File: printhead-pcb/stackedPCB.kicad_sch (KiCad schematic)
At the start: 5 parts, among them J13 Steckverbinder_Male_1

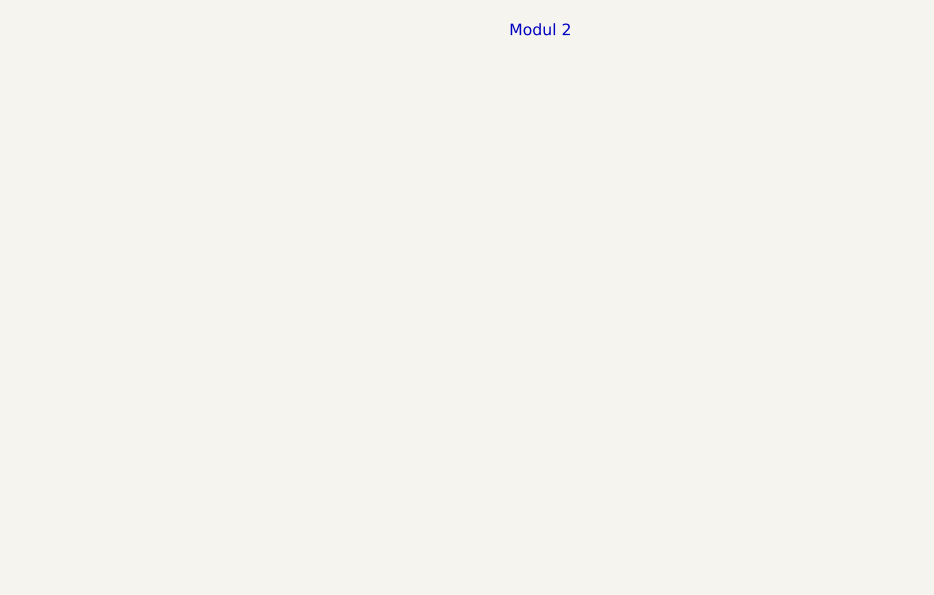
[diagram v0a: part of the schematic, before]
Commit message: prepared second module for tomorrow
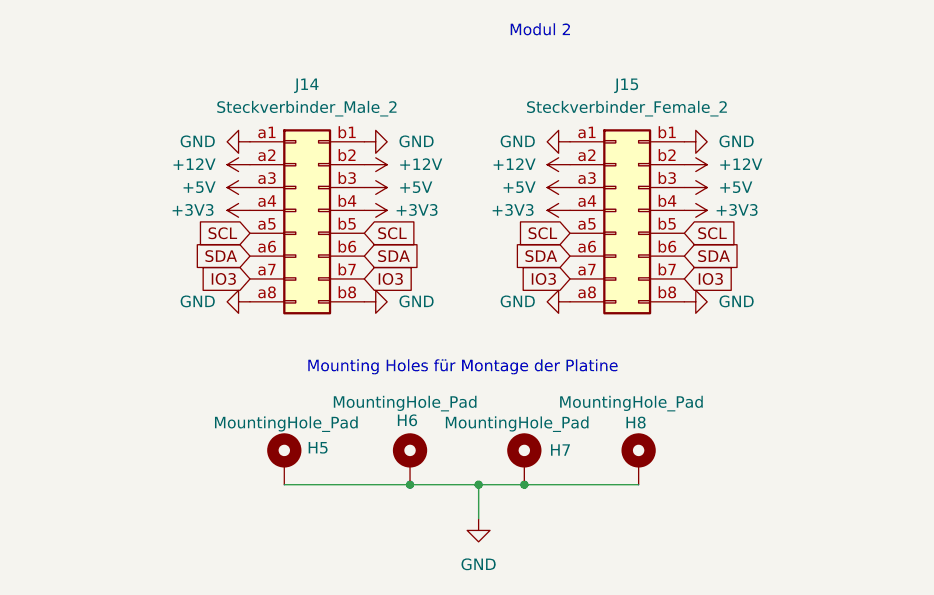
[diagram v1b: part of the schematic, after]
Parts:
- added H5, H6, H7, H8: MountingHole_Pad, MountingHole:MountingHole_2.2mm_M2_Pad_TopBottom, symbol Mechanical:MountingHole_Pad
- added J14: Steckverbinder_Male_2, CustomFotLibByJan:BF100-16-A-D-1-0640-L-C, symbol Connector_Generic:Conn_02x08_Row_Letter_First
- added J15: Steckverbinder_Female_2, CustomFotLibByJan:BF100-16-A-D-1-0640-L-C, symbol Connector_Generic:Conn_02x08_Row_Letter_First
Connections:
- net +12V: now also J14.a2 (Pin_a2), J14.b2 (Pin_b2), J15.a2 (Pin_a2), J15.b2 (Pin_b2)
- net +3V3: now also J14.a4 (Pin_a4), J14.b4 (Pin_b4), J15.a4 (Pin_a4), J15.b4 (Pin_b4)
- net +5V: now also J14.a3 (Pin_a3), J14.b3 (Pin_b3), J15.a3 (Pin_a3), J15.b3 (Pin_b3)
- net GND: now also H5.1, H6.1, H7.1, H8.1, J14.a1 (Pin_a1), J14.a8 (Pin_a8), J14.b1 (Pin_b1), J14.b8 (Pin_b8), J15.a1 (Pin_a1), J15.a8 (Pin_a8), J15.b1 (Pin_b1), J15.b8 (Pin_b8)
- net IO3: now also J14.a7 (Pin_a7), J14.b7 (Pin_b7), J15.a7 (Pin_a7), J15.b7 (Pin_b7)
- net SCL: now also J14.a5 (Pin_a5), J14.b5 (Pin_b5), J15.a5 (Pin_a5), J15.b5 (Pin_b5)
- net SDA: now also J14.a6 (Pin_a6), J14.b6 (Pin_b6), J15.a6 (Pin_a6), J15.b6 (Pin_b6)

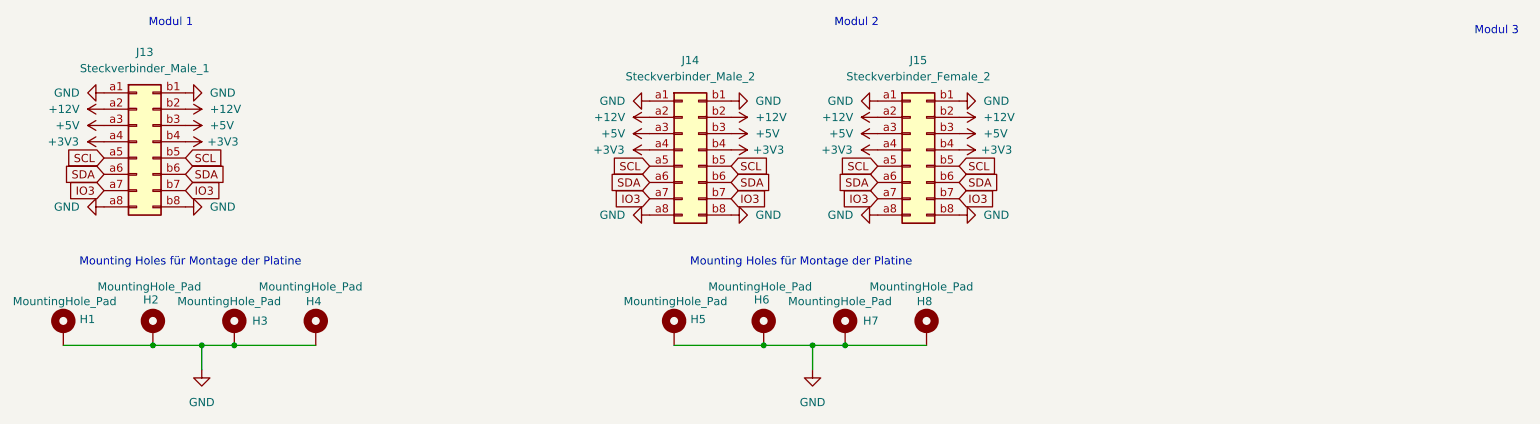
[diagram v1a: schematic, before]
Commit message: refractoring
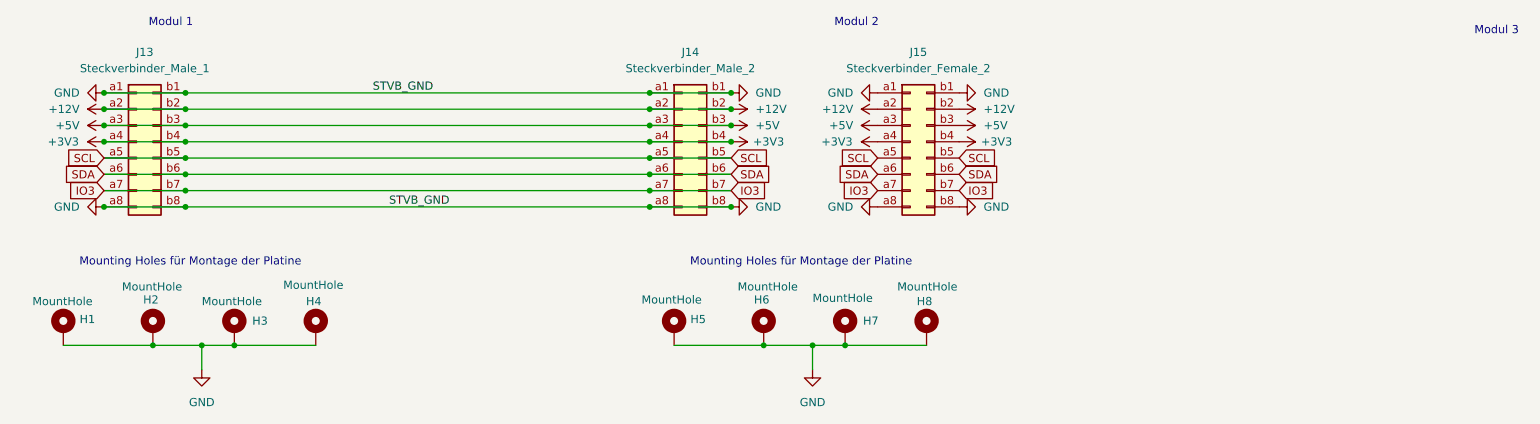
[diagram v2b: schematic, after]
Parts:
- H1, H2, H3, H4, H5, H6, H7, H8: value MountingHole_Pad -> MountHole
- J15: footprint CustomFotLibByJan:BF100-16-A-D-1-0640-L-C -> CustomFotLibByJan:BF030-16A-B1-0360-0277-0600-LB
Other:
- moved on the sheet: J14, J15

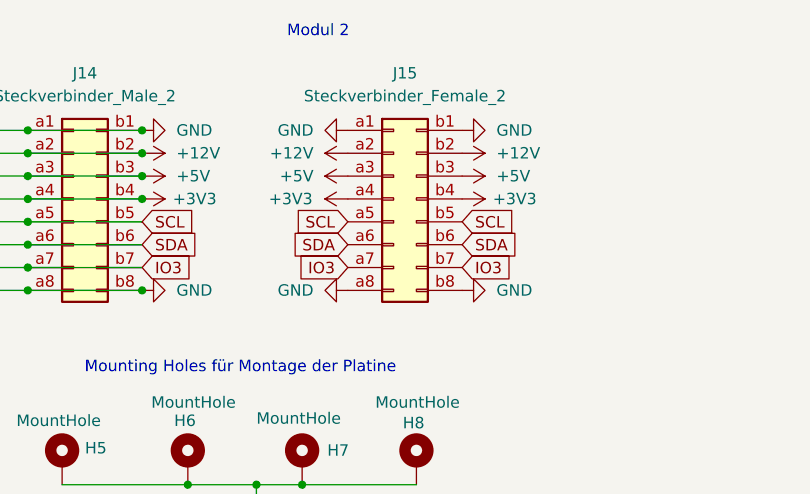
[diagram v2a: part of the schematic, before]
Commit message: unsaved changes
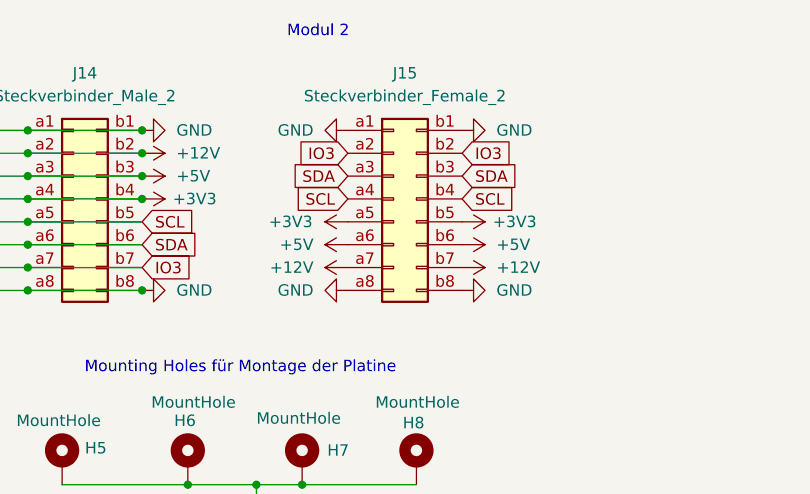
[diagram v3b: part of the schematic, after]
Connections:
- net +12V: now also J15.a7 (Pin_a7), J15.b7 (Pin_b7); no longer J15.a2 (Pin_a2), J15.b2 (Pin_b2)
- net +3V3: now also J15.a5 (Pin_a5), J15.b5 (Pin_b5); no longer J15.a4 (Pin_a4), J15.b4 (Pin_b4)
- net +5V: now also J15.a6 (Pin_a6), J15.b6 (Pin_b6); no longer J15.a3 (Pin_a3), J15.b3 (Pin_b3)
- net IO3: now also J15.a2 (Pin_a2), J15.b2 (Pin_b2); no longer J15.a7 (Pin_a7), J15.b7 (Pin_b7)
- net SCL: now also J15.a4 (Pin_a4), J15.b4 (Pin_b4); no longer J15.a5 (Pin_a5), J15.b5 (Pin_b5)
- net SDA: now also J15.a3 (Pin_a3), J15.b3 (Pin_b3); no longer J15.a6 (Pin_a6), J15.b6 (Pin_b6)

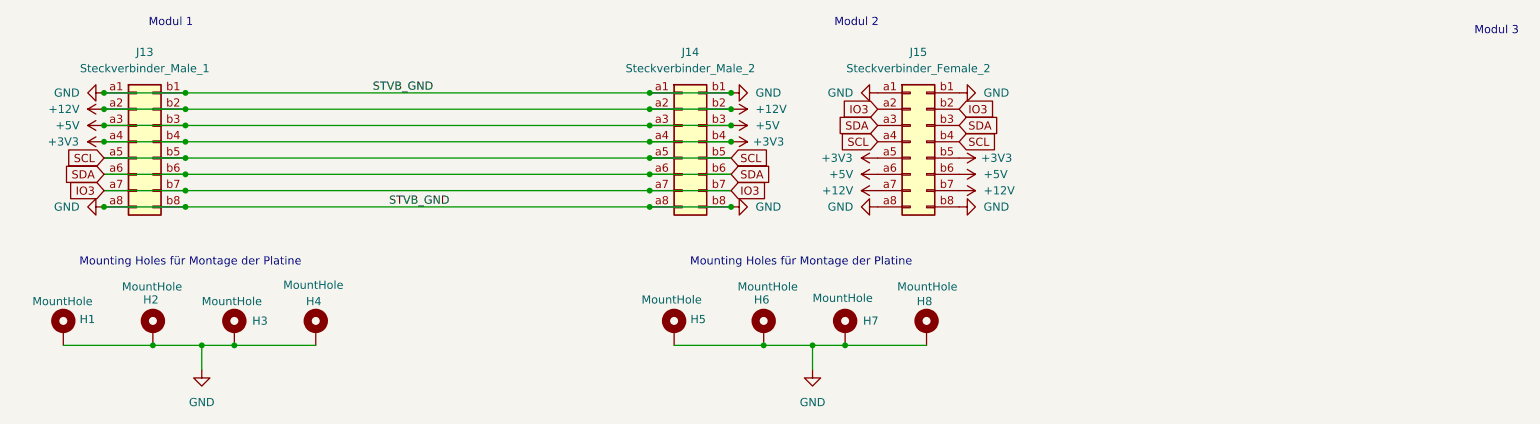
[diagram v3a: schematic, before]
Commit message: played around with nets and net classes
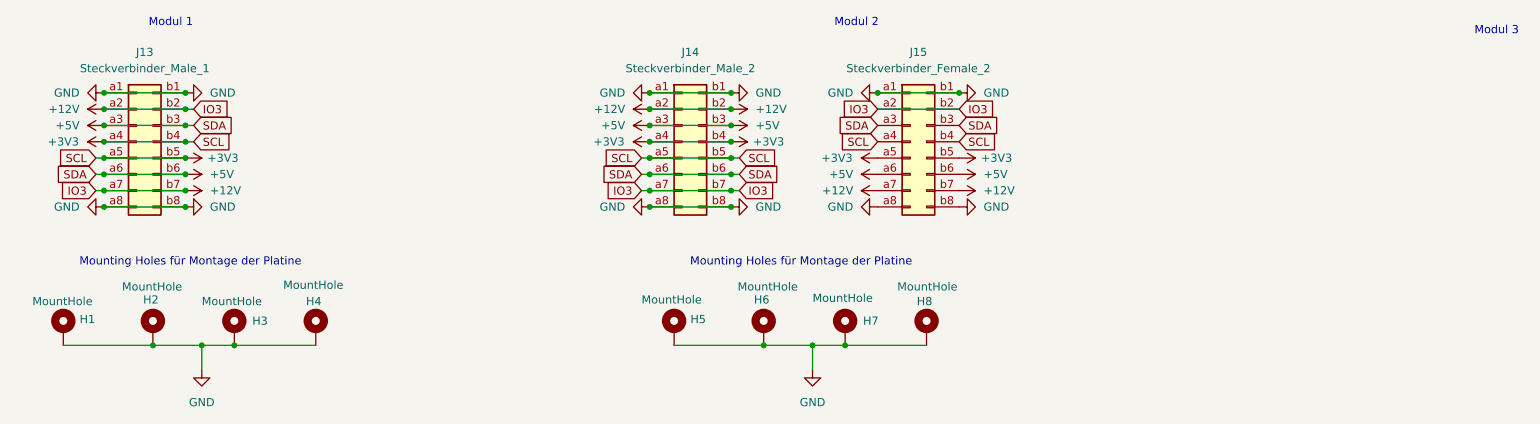
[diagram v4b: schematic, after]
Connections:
- net IO3 is gone; now on net +12V: J13.a7 (Pin_a7), J13.b7 (Pin_b7), J14.a7 (Pin_a7), J14.b7 (Pin_b7), J15.a2 (Pin_a2), J15.b2 (Pin_b2)
- net SCL is gone; now on net +3V3: J13.a5 (Pin_a5), J13.b5 (Pin_b5), J14.a5 (Pin_a5), J14.b5 (Pin_b5), J15.a4 (Pin_a4), J15.b4 (Pin_b4)
- net SDA is gone; now on net +5V: J13.a6 (Pin_a6), J13.b6 (Pin_b6), J14.a6 (Pin_a6), J14.b6 (Pin_b6), J15.a3 (Pin_a3), J15.b3 (Pin_b3)
